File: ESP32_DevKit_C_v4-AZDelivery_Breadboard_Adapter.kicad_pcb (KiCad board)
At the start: 4 copper layers, 133 x 29 mm, 9 parts, among them J1 Conn_01x19_Female, J2 Conn_01x19_Female, J3 Conn_01x18_Male, J4 Conn_01x18_Male, J5 Conn_01x04_Female

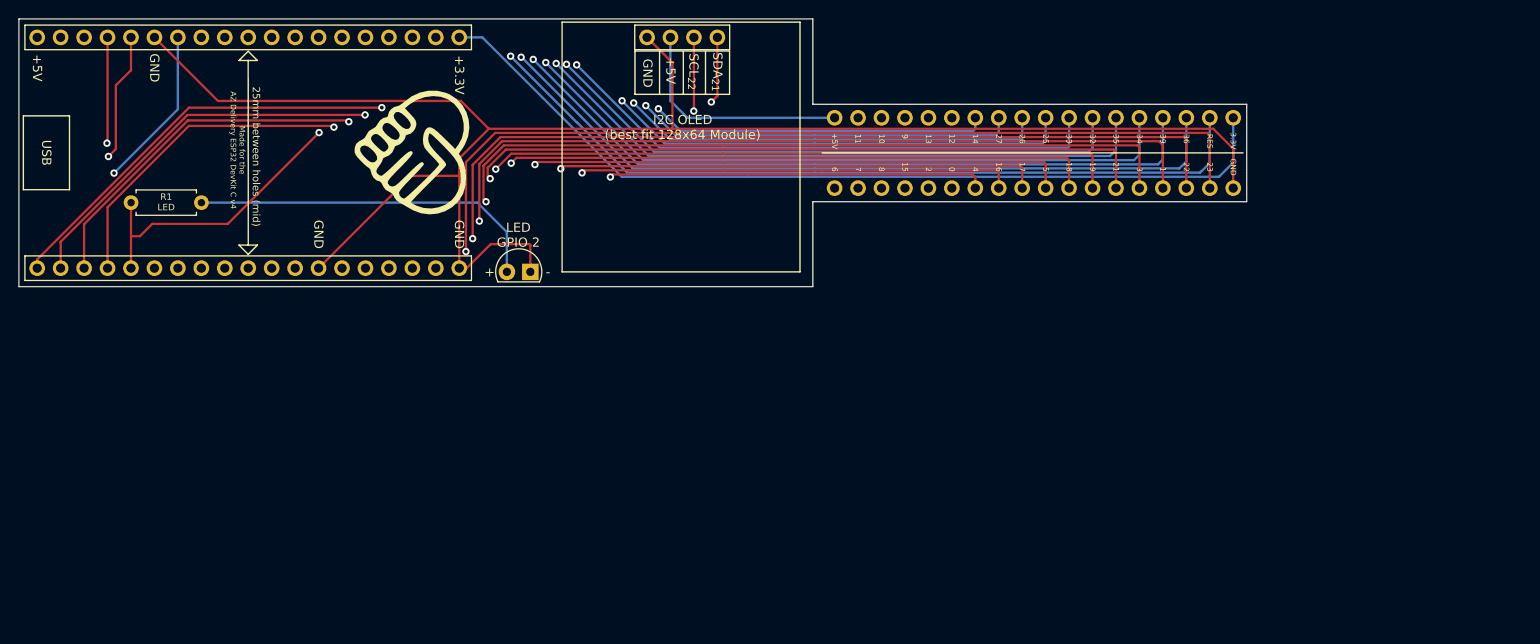
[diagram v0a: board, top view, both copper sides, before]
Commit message: update
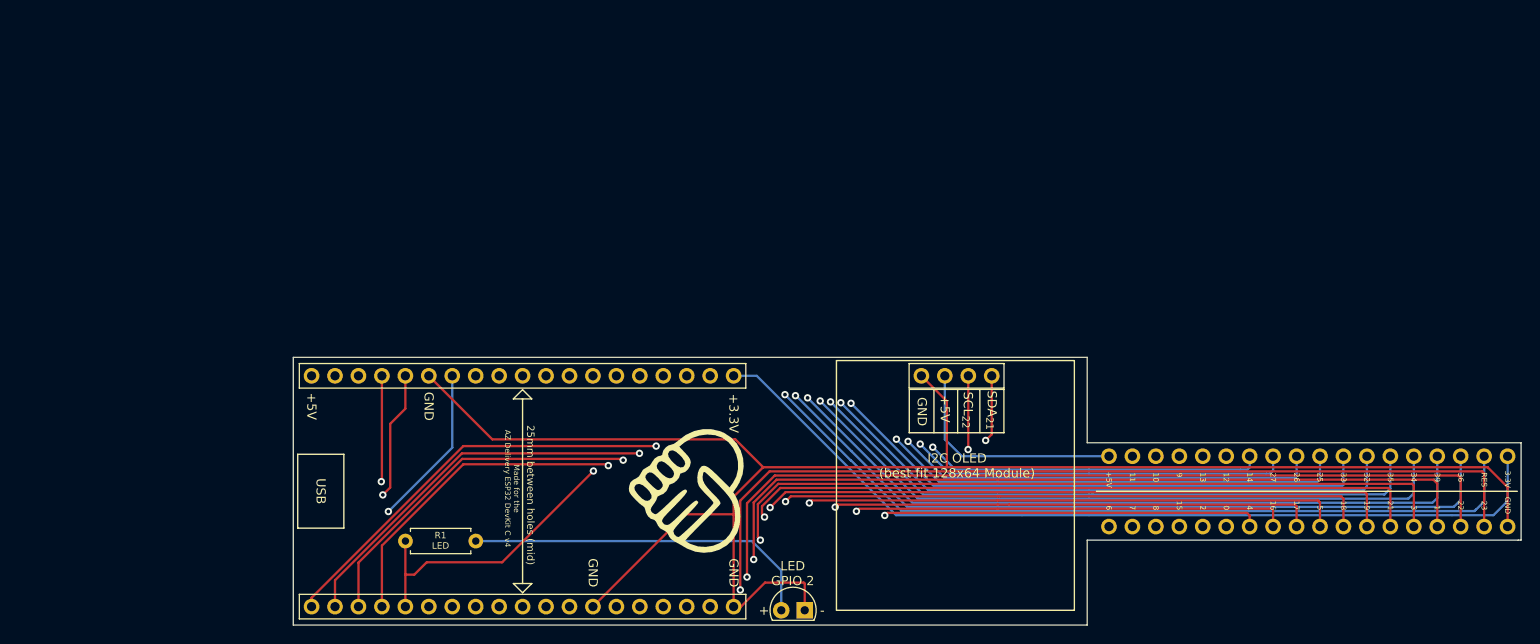
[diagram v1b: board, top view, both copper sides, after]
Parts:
- moved J1 47.2 mm to (151.6, 91.5)
- moved J5 47.2 mm to (172.0, 91.5)
- moved D1 47.2 mm to (159.3, 116.8)
- moved G*** 47.2 mm to (146.6, 103.9)
- moved J2 47.2 mm to (151.6, 116.5)
- moved J3 47.2 mm to (235.5, 100.2)
- moved J4 47.2 mm to (235.5, 107.8)
- moved R1 47.2 mm to (116.1, 109.3)
- moved G*** 47.2 mm to (137.6, 105.3)
